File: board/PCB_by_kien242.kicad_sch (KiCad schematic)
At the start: 55 parts, among them J1 VIN, J2 , J4 TC1, J6 SSR1, J7 SSR2, J8 SSR3, Q1 AO3407, Q4 IRLR2905Z, Q5 IRLR2905Z, Q6 IRLR2905Z, Q7 2N3904, Q8 2N3904, SW3 SW_RESET, SW4 SW_BOOT, U1 NCP1117-3.3_SOT223, U2 YAAJ_DCDC_StepDown_LM2596, U4 MAX31855KASA, U5 ESP32-WROOM-32, U6 CH340G, Y1 12mhz

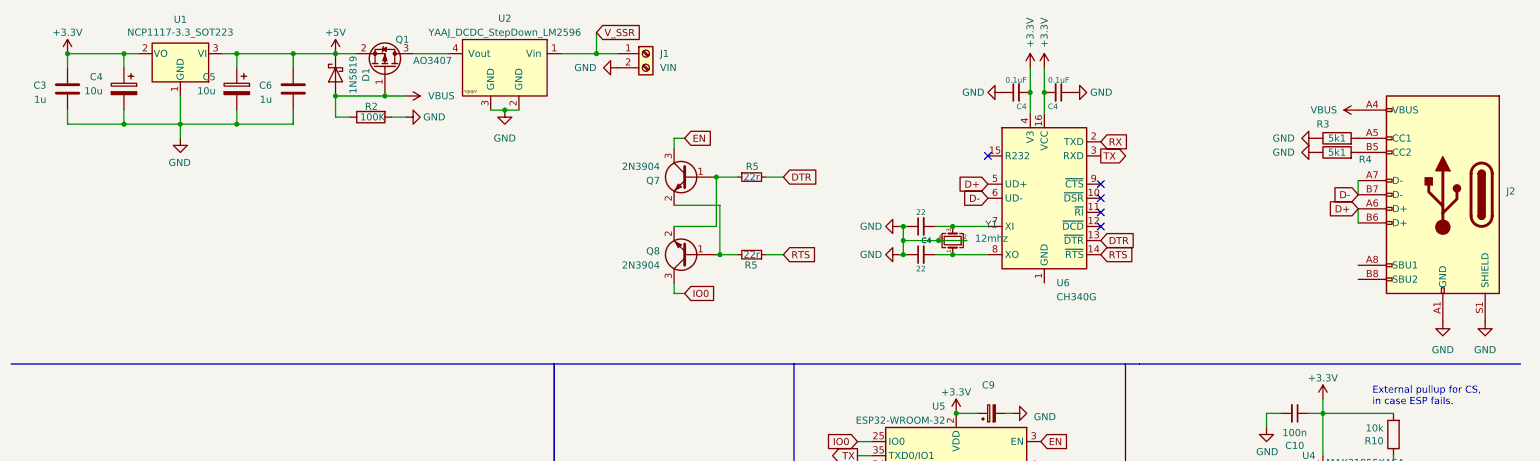
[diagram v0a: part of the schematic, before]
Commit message: Update
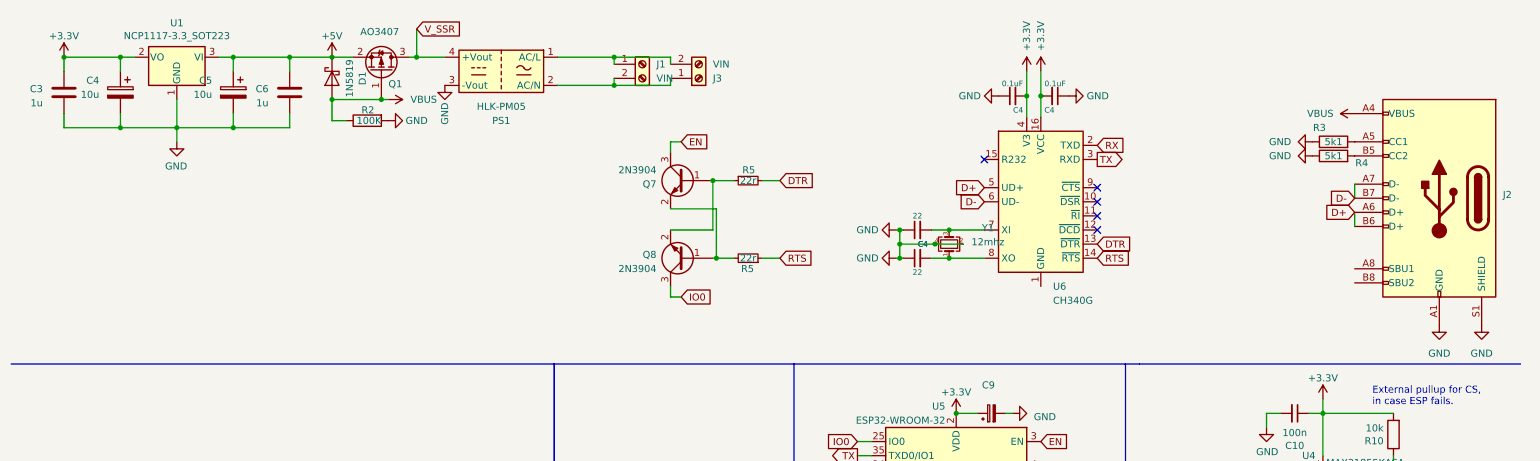
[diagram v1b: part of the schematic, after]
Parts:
- removed U2: YAAJ_DCDC_StepDown_LM2596, TerminalBlock_KF301:YAAJ_DCDC_StepDown_LM2596, symbol yaaj_dcdc_stepdown_lm2596:YAAJ_DCDC_StepDown_LM2596
- added J3: VIN, TerminalBlock:TerminalBlock_bornier-2_P5.08mm, symbol Connector:Screw_Terminal_01x02
- added PS1: HLK-PM05, Converter_ACDC:Converter_ACDC_Hi-Link_HLK-PMxx, symbol Converter_ACDC:HLK-PM09
- J1: footprint TerminalBlock_4Ucon:TerminalBlock_4Ucon_1x02_P3.50mm_Horizontal -> TerminalBlock:TerminalBlock_bornier-2_P5.08mm
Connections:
- net GND: now also PS1.3 (-Vout); no longer J1.2 (Pin_2)
- net V_SSR: now also Q1.3 (D), PS1.4 (+Vout); no longer J1.1 (Pin_1)
- new net: J1.1 (Pin_1), J3.2 (Pin_2), PS1.1 (AC/L)
- new net: J1.2 (Pin_2), J3.1 (Pin_1), PS1.2 (AC/N)
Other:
- moved on the sheet: C3, C4, C5, C6, D1, J1, J2, Q1, Q7, Q8, R2, R3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
